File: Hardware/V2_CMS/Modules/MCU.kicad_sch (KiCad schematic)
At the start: 2 parts, among them U15 ATmega328P-A

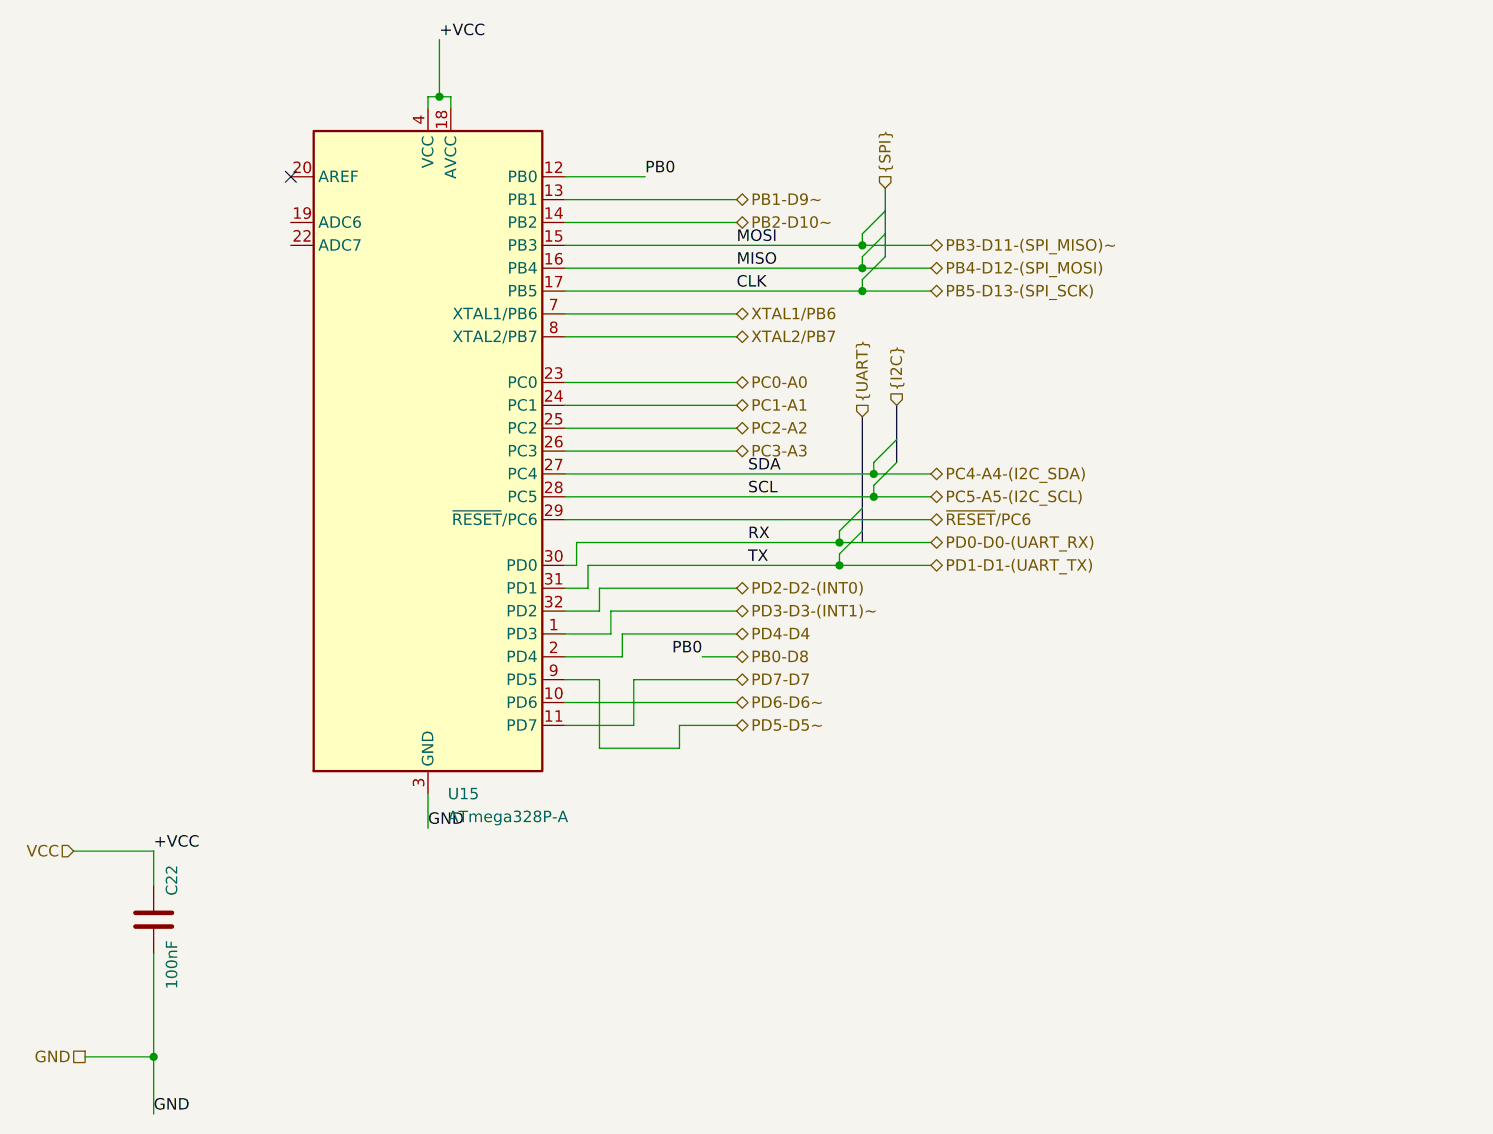
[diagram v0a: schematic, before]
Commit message: update of directory
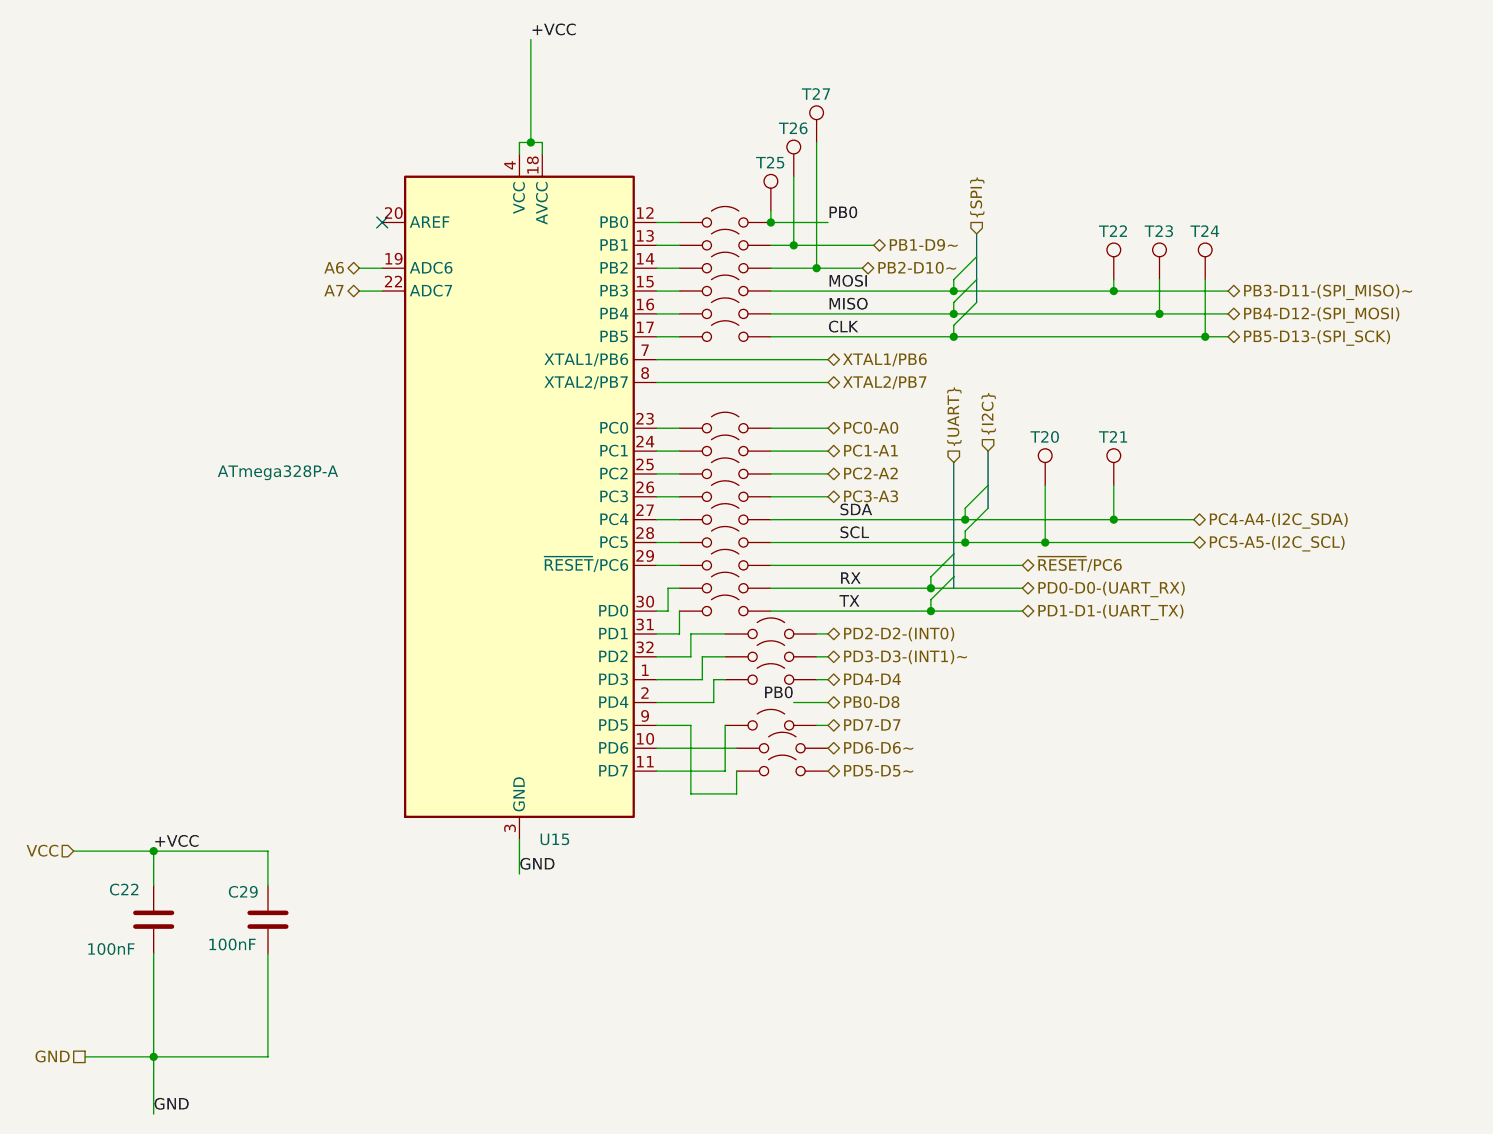
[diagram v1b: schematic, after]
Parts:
- added C29: 100nF, Capacitor_SMD:C_0603_1608Metric, symbol Device:C
- added JP10, JP11, JP12, JP13, JP14, JP15, JP16, JP17, JP18, JP19, JP2, JP20, JP21, JP22, JP23, JP24, JP25, JP26, JP27, JP28, JP9: Jumper_2_Open, Connector_PinHeader_1.27mm:PinHeader_1x02_P1.27mm_Vertical, symbol Jumper:Jumper_2_Open
- added T20, T21, T22, T23, T24, T25, T26, T27: TP, TestPoint:TestPoint_Pad_D1.0mm, symbol Connector:TestPoint
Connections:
- net GND: now also C29.1
- net PB0-D8: now also JP2.2 (B), T25.1; no longer U15.12 (PB0)
- net PB1-D9~: now also JP9.2 (B), T26.1; no longer U15.13 (PB1)
- net PB2-D10~: now also JP10.2 (B), T27.1; no longer U15.14 (PB2)
- net PB3-D11-(SPI_MISO)~: now also JP11.2 (B), T22.1; no longer U15.15 (PB3)
- net PB4-D12-(SPI_MOSI): now also JP12.2 (B), T23.1; no longer U15.16 (PB4)
- net PB5-D13-(SPI_SCK): now also JP13.2 (B), T24.1; no longer U15.17 (PB5)
- net PC0-A0: now also JP14.2 (B); no longer U15.23 (PC0)
- net PC1-A1: now also JP15.2 (B); no longer U15.24 (PC1)
- net PC2-A2: now also JP16.2 (B); no longer U15.25 (PC2)
- net PC3-A3: now also JP17.2 (B); no longer U15.26 (PC3)
- net PC4-A4-(I2C_SDA): now also JP18.2 (B), T21.1; no longer U15.27 (PC4)
- net PC5-A5-(I2C_SCL): now also JP19.2 (B), T20.1; no longer U15.28 (PC5)
- net PD0-D0-(UART_RX): now also JP21.2 (B); no longer U15.30 (PD0)
- net PD1-D1-(UART_TX): now also JP22.2 (B); no longer U15.31 (PD1)
- net PD2-D2-(INT0): now also JP23.2 (B); no longer U15.32 (PD2)
- net PD3-D3-(INT1)~: now also JP24.2 (B); no longer U15.1 (PD3)
- net PD4-D4: now also JP25.2 (B); no longer U15.2 (PD4)
- net PD5-D5~: now also JP28.2 (B); no longer U15.9 (PD5)
- net PD6-D6~: now also JP27.2 (B); no longer U15.10 (PD6)
- net PD7-D7: now also JP26.2 (B); no longer U15.11 (PD7)
- net VCC: now also C29.2
- net ~{RESET}/PC6: now also JP20.2 (B); no longer U15.29 (~{RESET}/PC6)
- net A6: now reaches U15.19 (ADC6)
- net A7: now reaches U15.22 (ADC7)
- new net: JP25.1 (A), U15.2 (PD4)
- new net: JP10.1 (A), U15.14 (PB2)
- new net: JP18.1 (A), U15.27 (PC4)
- new net: JP11.1 (A), U15.15 (PB3)
- new net: JP20.1 (A), U15.29 (~{RESET}/PC6)
- new net: JP19.1 (A), U15.28 (PC5)
- new net: JP9.1 (A), U15.13 (PB1)
- new net: JP28.1 (A), U15.9 (PD5)
- new net: JP27.1 (A), U15.10 (PD6)
- new net: JP2.1 (A), U15.12 (PB0)
- new net: JP22.1 (A), U15.31 (PD1)
- new net: JP24.1 (A), U15.1 (PD3)
- new net: JP26.1 (A), U15.11 (PD7)
- new net: JP12.1 (A), U15.16 (PB4)
- new net: JP13.1 (A), U15.17 (PB5)
- new net: JP14.1 (A), U15.23 (PC0)
- new net: JP15.1 (A), U15.24 (PC1)
- new net: JP16.1 (A), U15.25 (PC2)
- new net: JP17.1 (A), U15.26 (PC3)
- new net: JP21.1 (A), U15.30 (PD0)
- new net: JP23.1 (A), U15.32 (PD2)
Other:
- moved on the sheet: U15
